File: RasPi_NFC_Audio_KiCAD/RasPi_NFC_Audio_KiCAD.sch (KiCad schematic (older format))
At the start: 5 parts, among them P1 Conn_02x20_Odd_Even

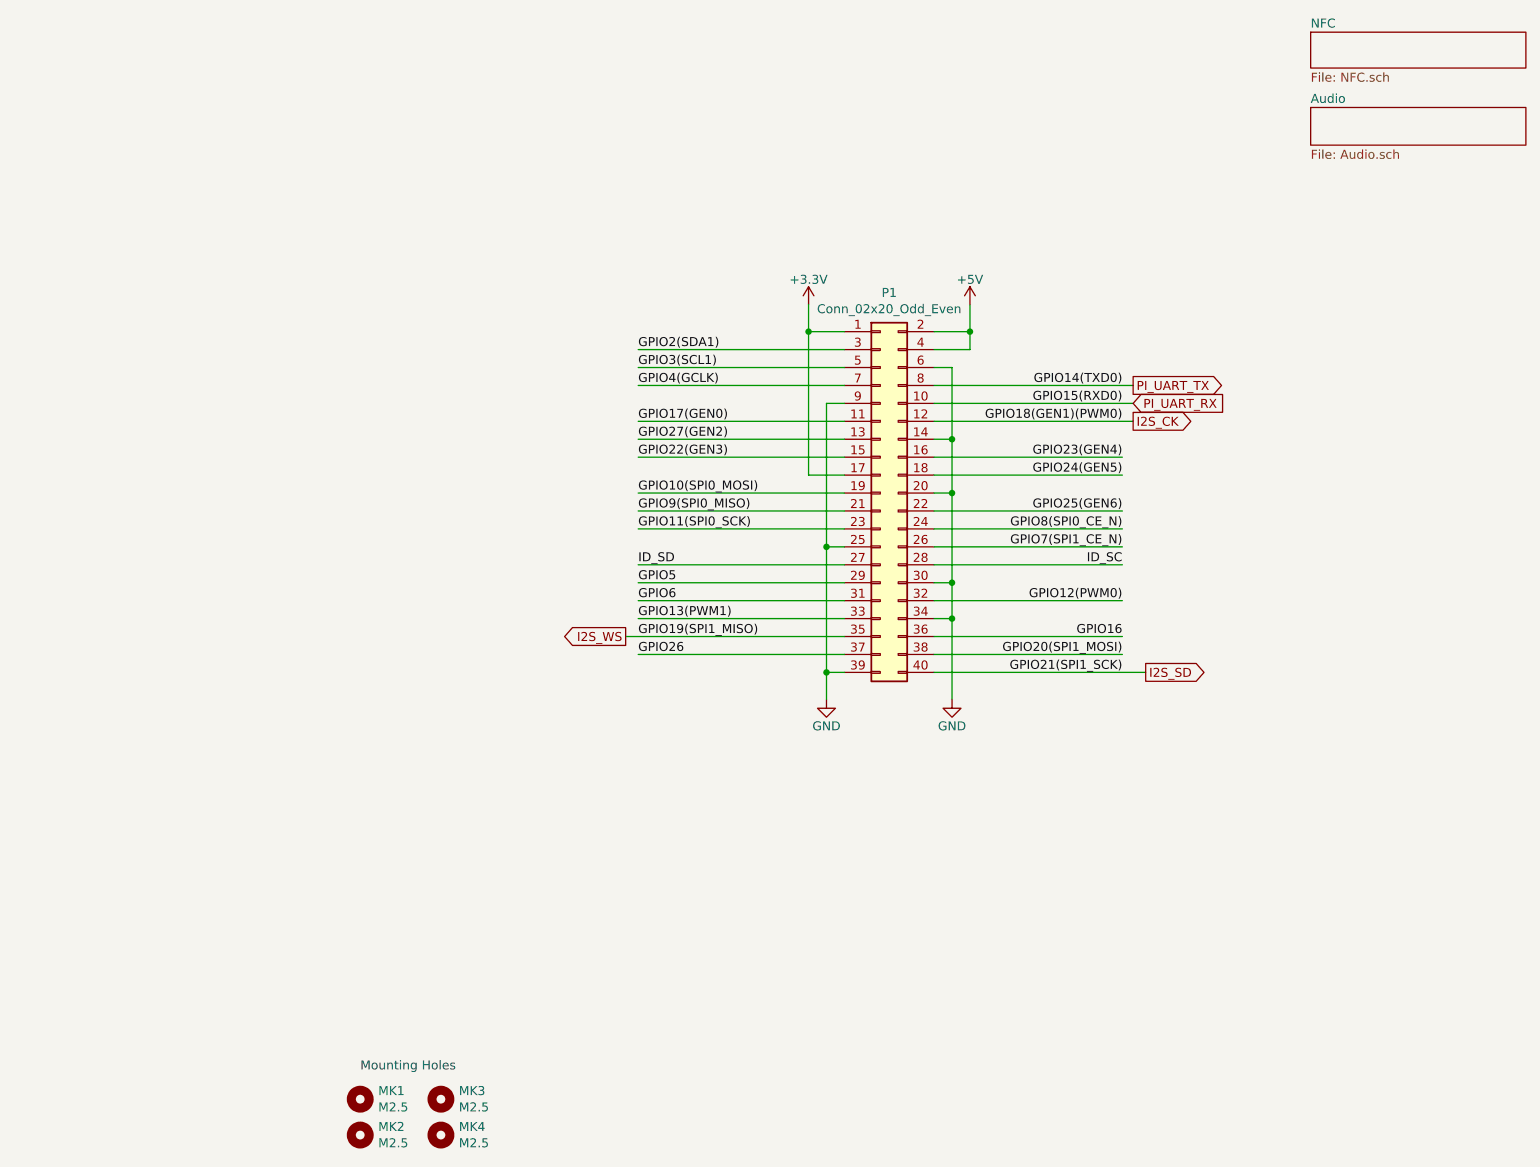
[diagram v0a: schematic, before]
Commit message: Schematic update
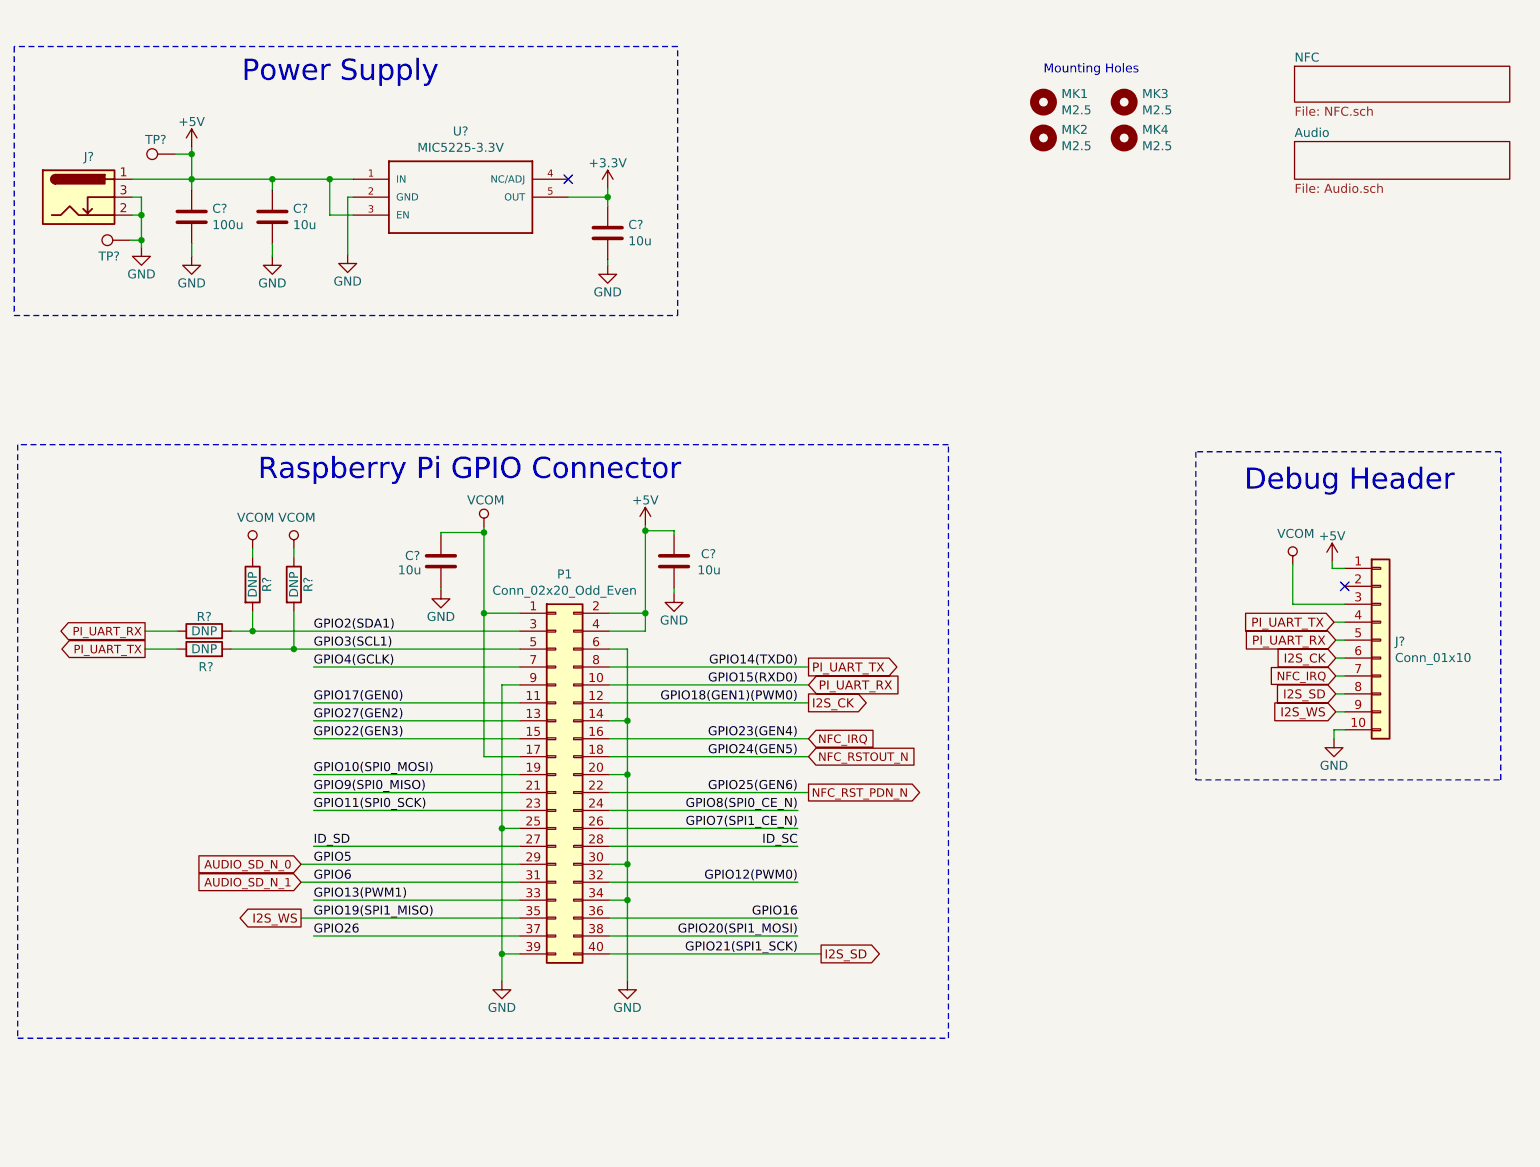
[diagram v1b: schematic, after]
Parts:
- added C?: 100u, symbol Device:C
- added C? (x4): 10u, symbol Device:C
- added J?: Conn_01x10, symbol Connector_Generic:Conn_01x10
- added J?: Barrel_Jack_Switch, symbol Connector:Barrel_Jack_Switch
- added R? (x4): DNP, Resistors_SMD:R_0603_HandSoldering, symbol Device:R
- added TP? (x2): TestPoint, symbol Connector:TestPoint
- added U?: MIC5225-3.3V, SOT95P280X130-5N, symbol MIC5225:MIC5225
- P1: DigiKey (none) -> 952-1837-ND; Part # (none) -> M20-7831046
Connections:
- net +3V3: now also C?.1, U?.5 (OUT); no longer P1.1 (Pin_1), P1.17 (Pin_17)
- net +5V: now also C?.1, C?.1, C?.1, J?.1, J?.1 (Pin_1), TP?.1, U?.1 (IN), U?.3 (EN)
- net GND: now also C?.2, C?.2, C?.2, C?.2, C?.2, J?.10 (Pin_10), J?.2, J?.3, TP?.1, U?.2 (GND)
- net GPIO2(SDA1): now also R?.2, R?.2
- net GPIO3(SCL1): now also R?.2, R?.2
- net I2S_CK: now also J?.6 (Pin_6)
- net I2S_SD: now also J?.8 (Pin_8)
- net I2S_WS: now also J?.9 (Pin_9)
- net PI_UART_RX: now also J?.5 (Pin_5), R?.1
- net PI_UART_TX: now also J?.4 (Pin_4), R?.1
- net GPIO23(GEN4) renamed NFC_IRQ
- net NFC_IRQ: now also J?.7 (Pin_7)
- net GPIO24(GEN5) renamed NFC_RSTOUT_N
- net GPIO25(GEN6) renamed NFC_RST_PDN_N
- net GPIO5 renamed AUDIO_SD_N_0
- net GPIO6 renamed AUDIO_SD_N_1
- new net VCOM: C?.1, J?.3 (Pin_3), P1.1 (Pin_1), P1.17 (Pin_17), R?.1, R?.1
- no-connect marks 0 -> 2
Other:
- note added: "Debug Header"
- note added: "Power Supply"
- note added: "Raspberry Pi GPIO Connector"
- moved on the sheet: MK1, MK2, MK3, MK4, P1
